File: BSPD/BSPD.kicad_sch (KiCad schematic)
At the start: 61 parts, among them J1 DT13-48PABCD-R015, K1 Latching Relay, K2 Latching Relay, Q2 STS6NF20V, Q3 STS6NF20V, Q4 STS6NF20V, U1 LM7805CT, U10 DK1A1B-12V, U12 LM555N, U13 LM7805CT, U14 ISO1050DUB, U15 LM7809_TO220, U17 NAND, U2 NSL-32, U2 OP AMP, U3 OP AMP, U4 NUCLEO-L432KC, U5 2x4 OR GATE, U6 LM555N, U8 NAND, U9 AND GATE

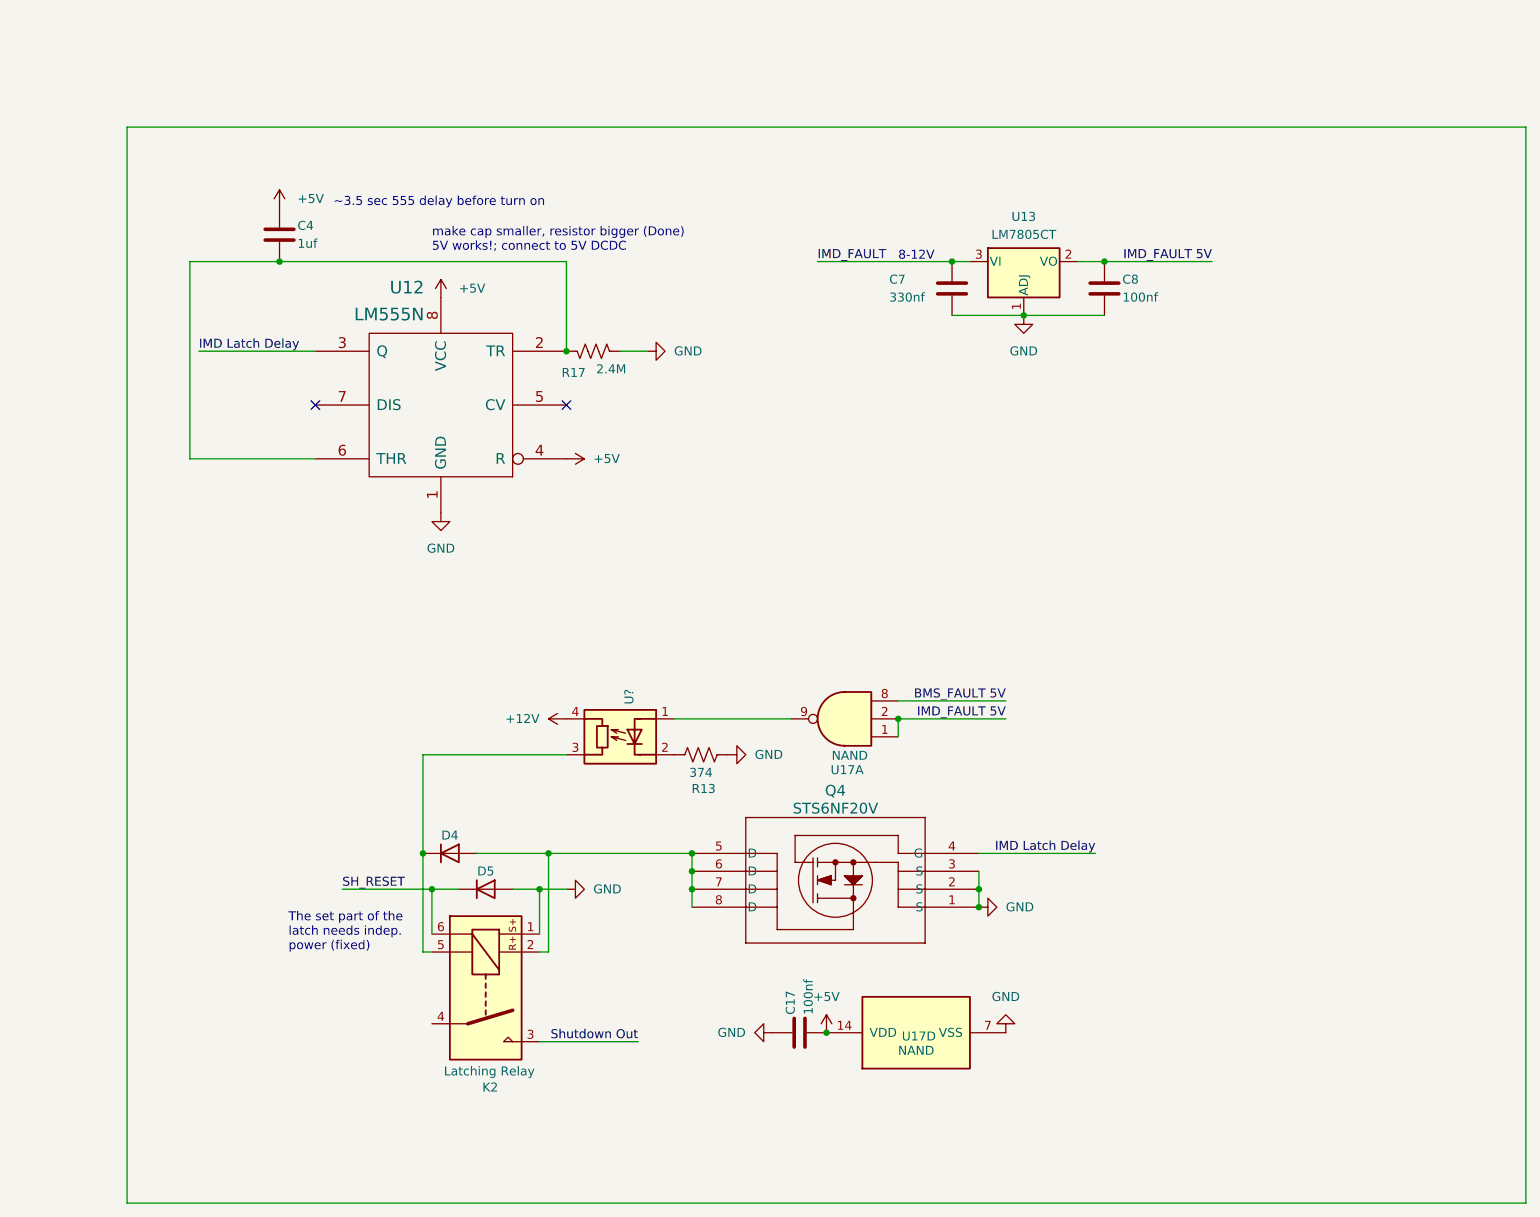
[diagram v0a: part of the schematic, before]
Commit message: cleared acc stuff
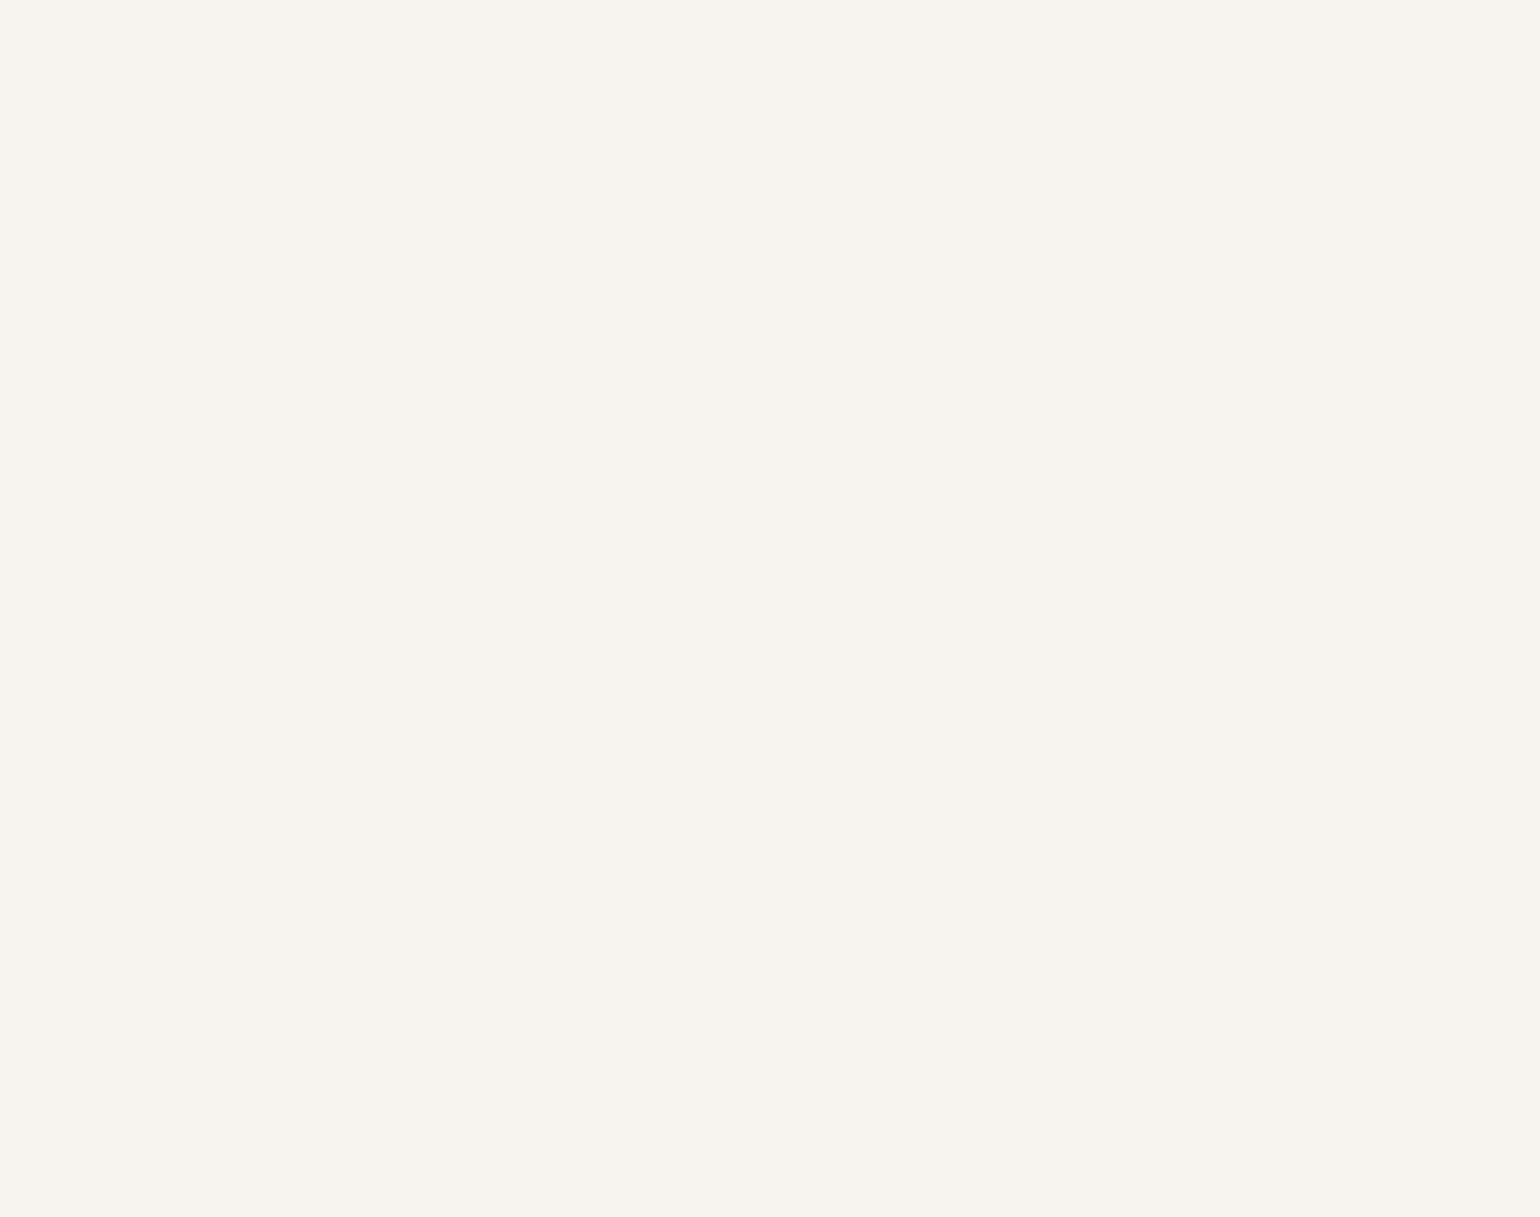
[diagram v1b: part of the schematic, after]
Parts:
- removed C17, C8: 100nf, Capacitor_SMD:C_0805_2012Metric_Pad1.18x1.45mm_HandSolder, symbol Device:C
- removed C4: 1uf, Capacitor_SMD:C_0805_2012Metric_Pad1.18x1.45mm_HandSolder, symbol Device:C
- removed C7: 330nf, Capacitor_SMD:C_0805_2012Metric_Pad1.18x1.45mm_HandSolder, symbol Device:C
- removed D4, D5: D, Diode_SMD:D_2010_5025Metric_Pad1.52x2.65mm_HandSolder, symbol Device:D
- removed K2: Latching Relay, 1FS_2_Global_Footprint_Library:Omron G6BK-1114P-US, symbol 1_Personal_FS_Library:G6BK-1114P-US
- removed Q4: STS6NF20V, 1FS_2_Global_Footprint_Library:SO-8_STM, symbol 1_ACC_BOARD:STS6NF20V
- removed R13: 374, Resistor_SMD:R_0805_2012Metric_Pad1.20x1.40mm_HandSolder, symbol Device:R_US
- removed R17: 2.4M, Resistor_SMD:R_0805_2012Metric_Pad1.20x1.40mm_HandSolder, symbol Device:R_US
- removed U12: LM555N, Package_DIP:DIP-8_W7.62mm, symbol 2FS-1_Symbol Library:LM555N
- removed U13: LM7805CT, Package_TO_SOT_THT:TO-220-3_Vertical, symbol Regulator_Linear:LM317_TO-252
- removed U17: NAND, Package_DIP:DIP-14_W7.62mm, symbol 4xxx:4023
- removed U?: NSL-32, 1FS_2_Global_Footprint_Library:OptoCoupler 6-SOP, symbol Isolator:NSL-32
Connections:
- no-connect marks 46 -> 44
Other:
- note removed: "8-12V"
- note removed: "~3.5 sec 555 delay before turn on"
